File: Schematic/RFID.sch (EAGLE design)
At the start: 14 parts, among them IC1 B82450A1084C000, U1 HTRC11001T/02EE,11

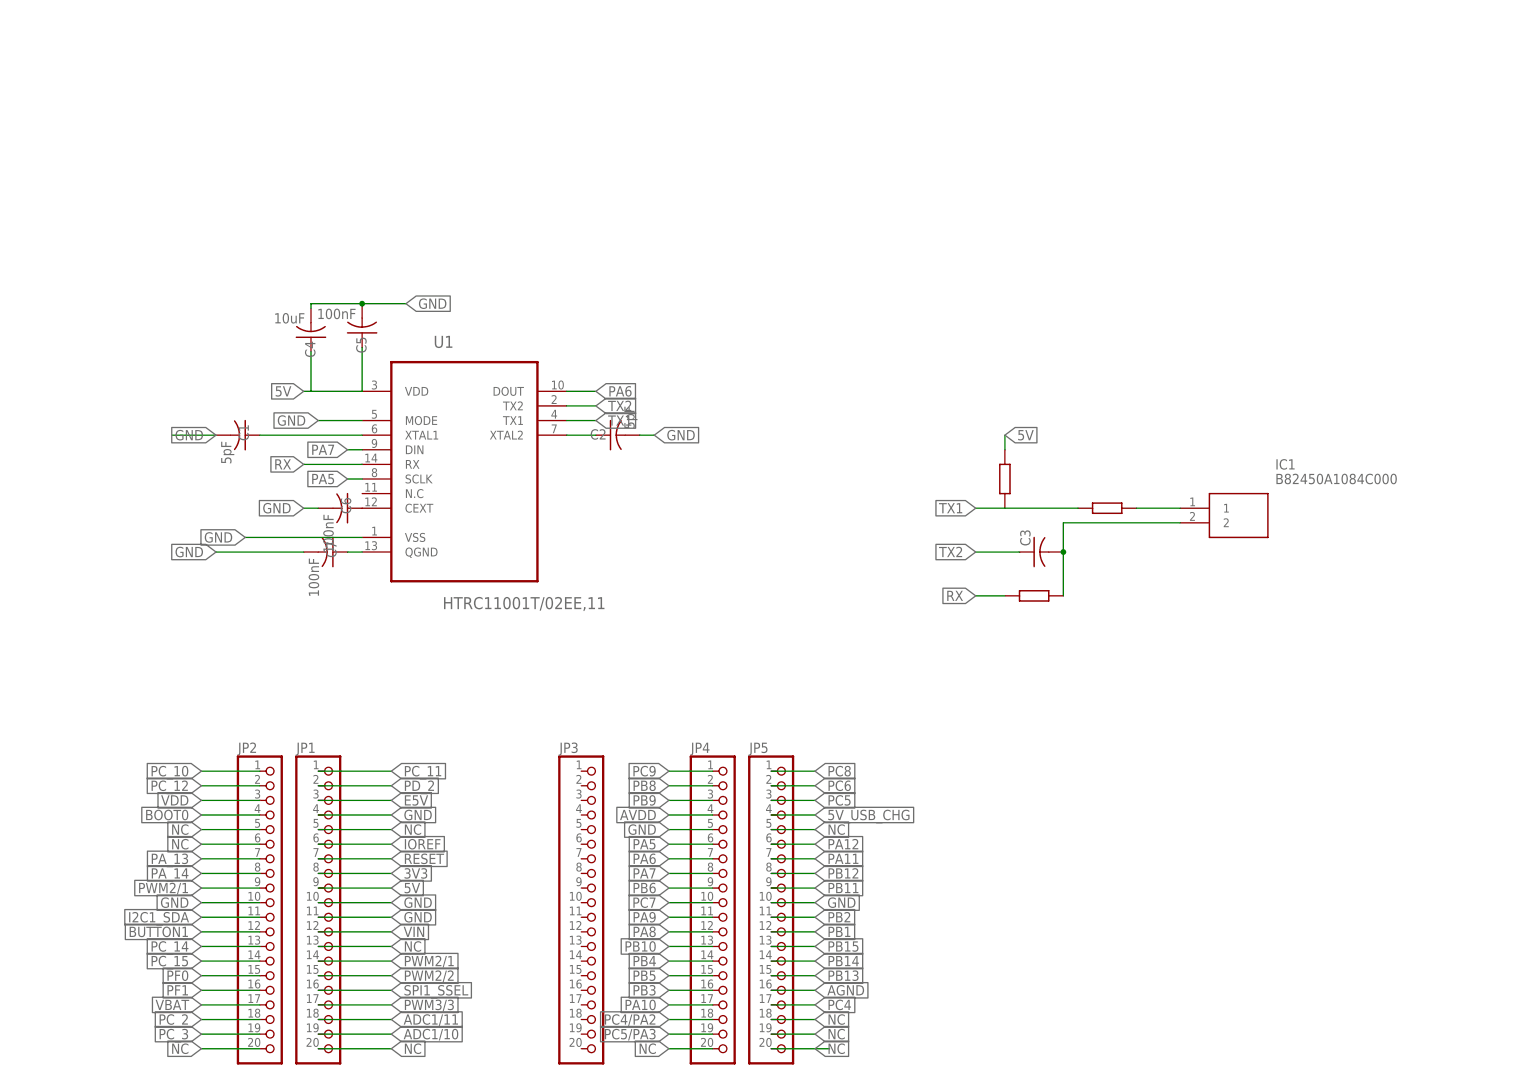
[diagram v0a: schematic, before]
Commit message: Aesthetics improved
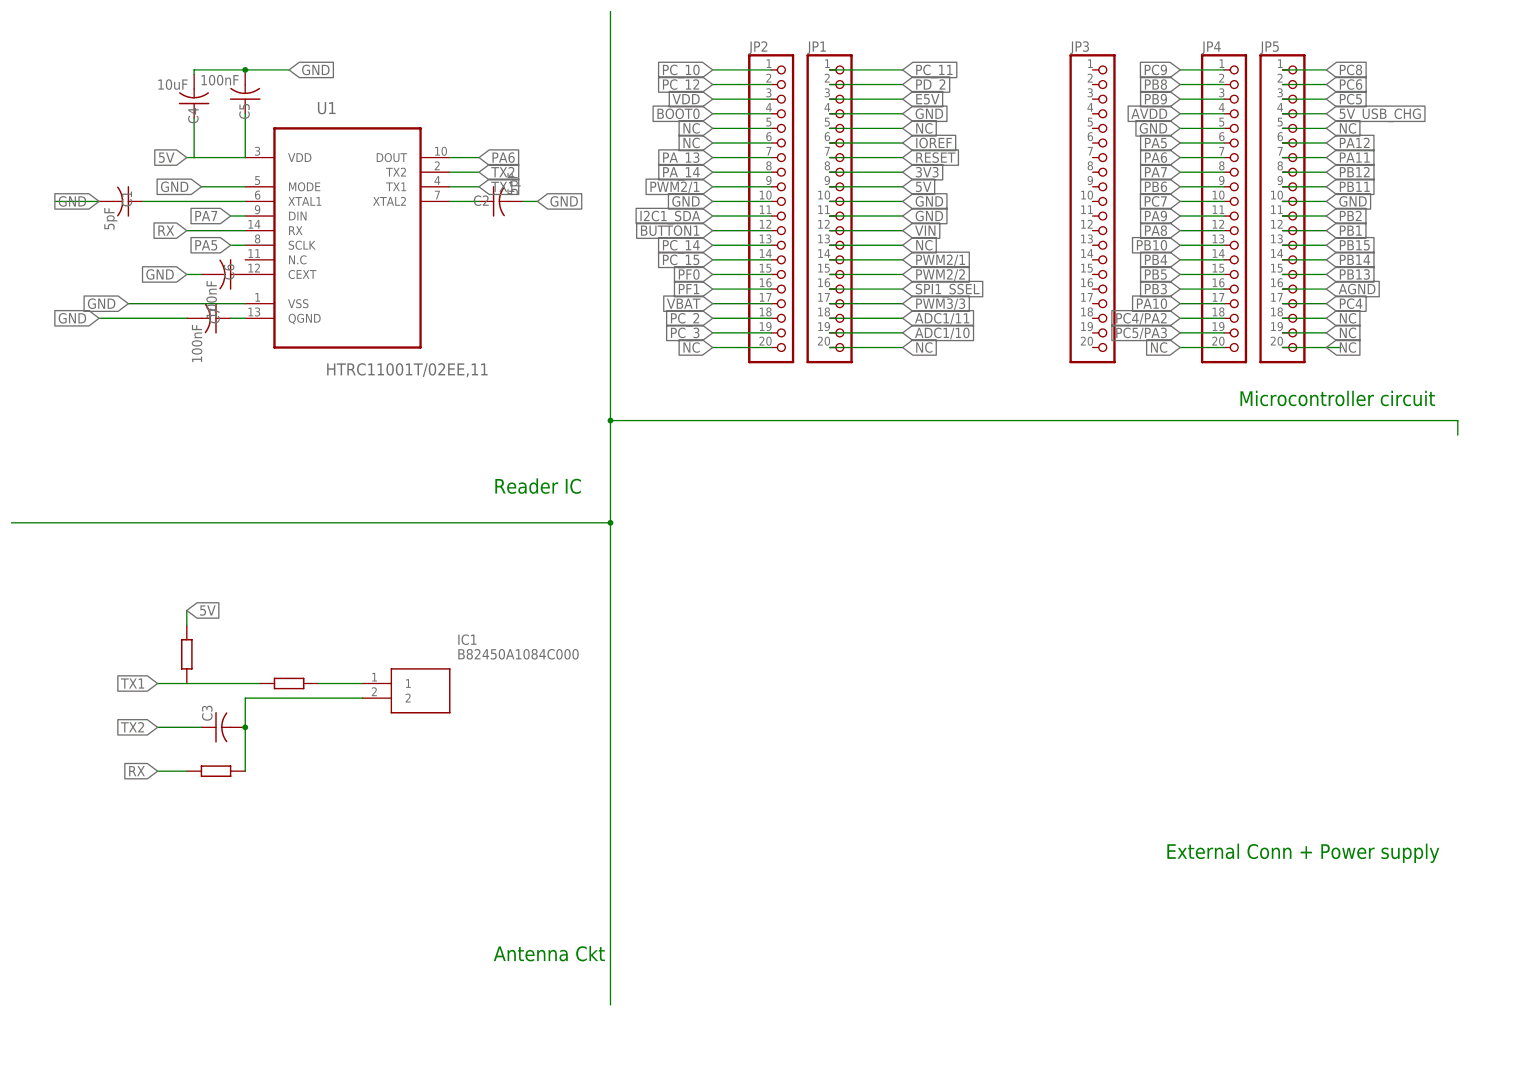
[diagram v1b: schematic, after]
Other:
- note added: "Antenna Ckt"
- note added: "External Conn + Power supply"
- note added: "Microcontroller circuit"
- note added: "Reader IC"
- moved on the sheet: C1, C2, C3, C4, C5, C6, C7, IC1, JP1, JP2, JP3, JP4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
